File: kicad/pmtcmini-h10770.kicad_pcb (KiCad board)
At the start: 2 copper layers, 19.5 x 39.1 mm, 34 parts, among them J1 Conn_01x03, J2 Conn_01x05, J3 10104110-0001LF, J4 DROK_Voltage_Converter, U1 MAX6106EUR-T, U2 MAX5214GUAT, U3 STM32F042F6P6, U4 ADP7118AUJZ-3.3-R7, U5 TPS22810-Q1, U6 ADP7118AUJZ-3.3-R7

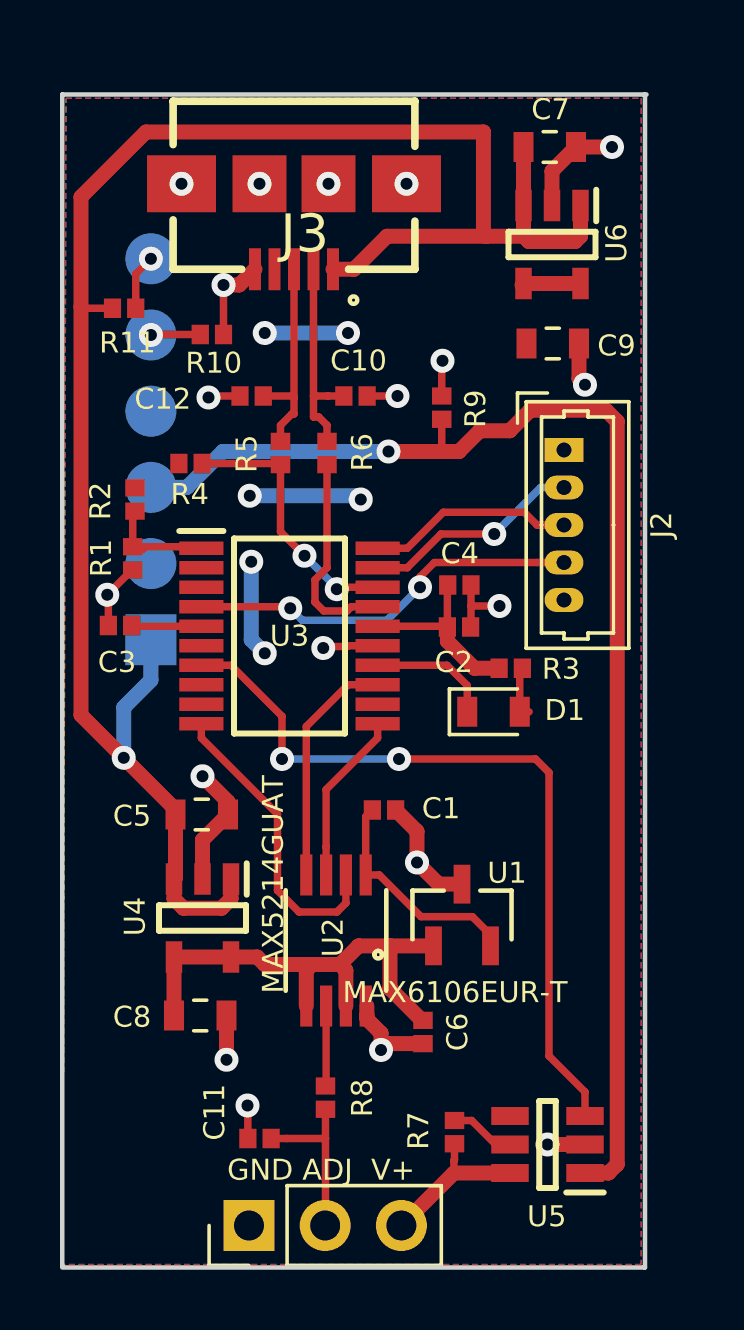
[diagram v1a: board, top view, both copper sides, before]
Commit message: rework progress
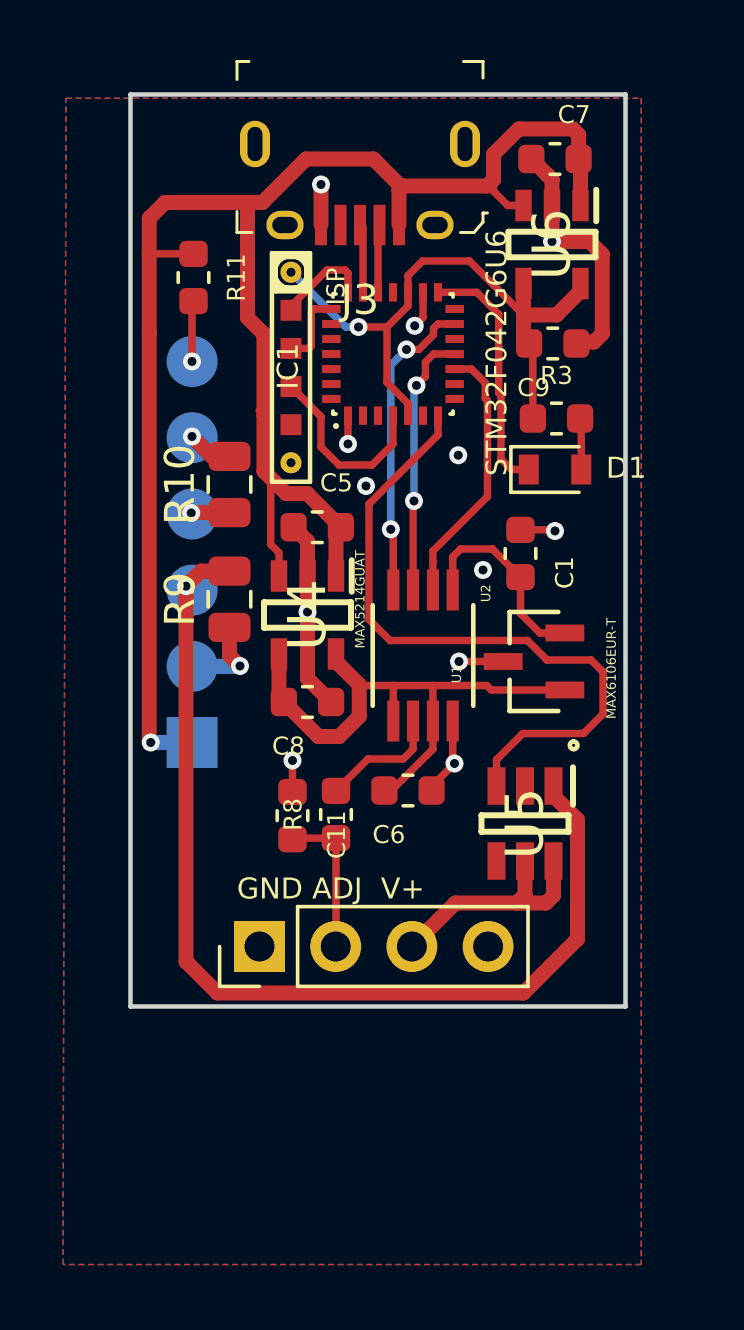
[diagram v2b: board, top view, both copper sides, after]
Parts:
- removed C10, C12: 47pF, Capacitor_SMD:C_0402_1005Metric
- removed C2: 1uF, Capacitor_SMD:C_0402_1005Metric
- removed C3, C4: 0.1uF, Capacitor_SMD:C_0402_1005Metric
- removed R1, R4: 1.5k, Resistor_SMD:R_0402_1005Metric
- removed R2, R7: 0, Resistor_SMD:R_0402_1005Metric
- removed R5, R6: 22, Resistor_SMD:R_0402_1005Metric
- removed U3: STM32F042F6P6, STM32F042F6P6:SOP65P640X120-20N
- added IC1: STM32F042G6U6, libraries:QFN50P400X400X60-28N, F.Cu at (135.8, 62.2)
- C1, C11, C6: footprint Capacitor_SMD:C_0402_1005Metric -> libraries:C_0603_1608Metric
- C5, C7, C8, C9: footprint Capacitor_SMD:C_0603_1608Metric -> libraries:C_0603_1608Metric
- J1: value Conn_01x03 -> Conn_01x04; footprint Connector_PinHeader_2.54mm:PinHeader_1x03_P2.54mm_Vertical -> libraries:PinHeader_1x04_P2.54mm_Vertical
- J2: footprint Connector_Molex:Molex_PicoBlade_53047-1010_1x05_P1.25mm_Vertical -> libraries:POGO_ISP
- J3: value 10104110-0001LF -> 10118194-0001LF; footprint 10104110-0001LF:10104110-0001LF -> libraries:USB_Micro_B_Female_10118194-0001LF
- R10, R9: footprint Resistor_SMD:R_0402_1005Metric -> libraries:R_0805_2012Metric
- R11, R8: footprint Resistor_SMD:R_0402_1005Metric -> libraries:R_0603_1608Metric
- R3: value 330 -> 1.5k; footprint Resistor_SMD:R_0402_1005Metric -> libraries:R_0603_1608Metric
- U4, U6: footprint ADP7118AUJZ-3.3-R7:SOT95P280X100-5N -> libraries:SOT95P280X100-5N
- moved C8 11.0 mm to (132.9, 73.8)
- moved C11 10.8 mm to (132.4, 77.6), turned to 90 degrees
- moved U5 10.7 mm to (140.2, 77.9), turned to 270 degrees
- moved U4 10.7 mm to (132.9, 71.0)
- moved C5 10.3 mm to (133.2, 68.0), turned to 180 degrees
- moved U2 9.93 mm to (136.8, 72.3)
- moved C1 9.69 mm to (140.0, 68.9), turned to 90 degrees
- moved R9 9.53 mm to (130.3, 70.4), turned to 90 degrees
- moved J2 9.51 mm to (132.3, 62.7), turned to 90 degrees
- moved R8 9.44 mm to (133.8, 77.6)
- moved J1 9.31 mm to (131.3, 82.0)
- moved U1 8.78 mm to (140.4, 72.5), turned to 90 degrees
- moved R3 8.46 mm to (141.2, 64.4)
- moved D1 8.33 mm to (141.2, 66.1)
- moved C6 8.07 mm to (136.2, 76.8), turned to 0 degrees
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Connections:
- net /V+ renamed /+12V
- net Net-(J4-Pad5) renamed /-12V
- J2 pad 5: GND -> Net-(J2-Pad5)
- U2 pad 2: /\CS -> /~CS
- U5 pad 5: Net-(R7-Pad1) -> /PMT_VDD
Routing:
- net /\CS: track 10.2 -> 0.00 mm
- net /+12V: track 43.8 -> 34.0 mm
- net Net-(R4-Pad1): track 8.95 -> 0.00 mm, vias 2 -> 0
- net /~CS: track 0.00 -> 8.90 mm
- net /RESET: track 13.5 -> 6.31 mm, vias 2 -> 0
- net Net-(R6-Pad2): track 7.02 -> 0.00 mm
- net /SWCLK: track 6.89 -> 2.55 mm
- net /USBM: track 6.51 -> 2.27 mm
- net /SWDIO: track 7.45 -> 3.23 mm, vias 1 -> 0
- net /USBP: track 6.48 -> 2.29 mm
- net /LED: track 4.14 -> 8.25 mm
- net Net-(R1-Pad1): track 3.61 -> 0.00 mm
- net +3V3: track 17.6 -> 21.1 mm, vias 6 -> 1
- net +3.3VA: track 16.9 -> 20.3 mm
- net VBUS: track 63.6 -> 60.3 mm
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- added copper zone on F.Cu, net GND
- removed copper zone on F.Cu, net +3V3
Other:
- board size 19.5 x 39.1 mm -> 16.5 x 30.4 mm
- rule pad_to_mask_clearance: 0.2 -> 0
- board text added: "PMTCMini H10770 Rev B"
- board text removed: "Eben Olson 2018"
- board text removed: "PMTCMini H10770 Rev A"
